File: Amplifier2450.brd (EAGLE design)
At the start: 28.2 x 35.5 mm, 17 parts, among them X1 SMA-142-0701-801/806, X2 SMA-142-0701-801/806

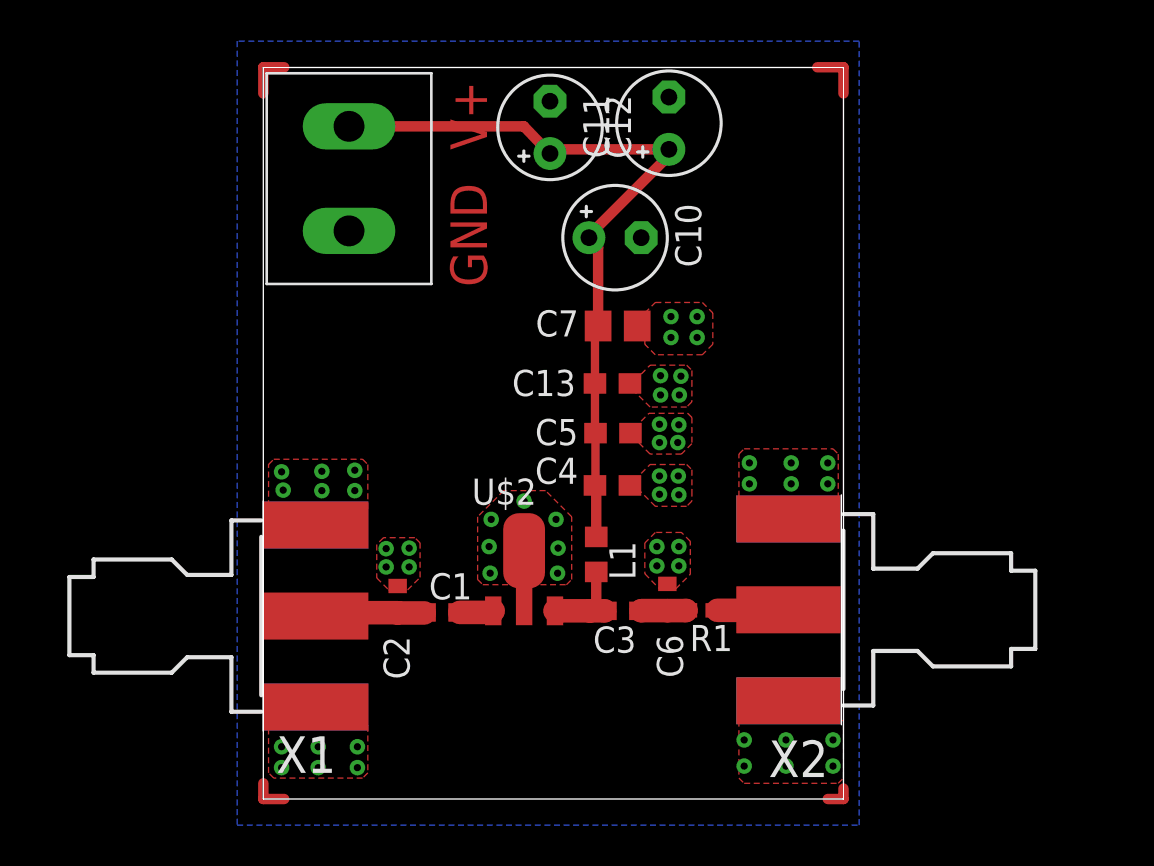
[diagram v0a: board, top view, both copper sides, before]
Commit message: (Tobias): made finishing touches to the design
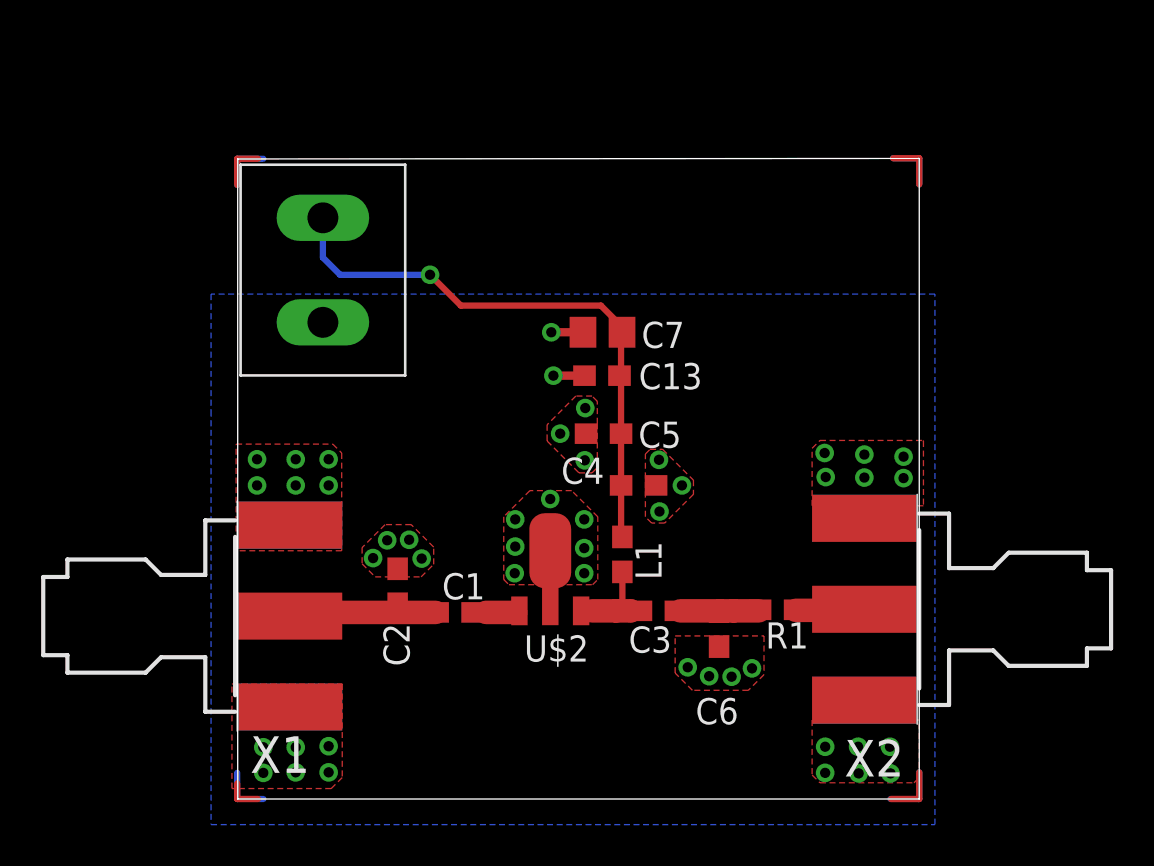
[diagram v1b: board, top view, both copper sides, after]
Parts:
- removed C10, C11, C12: 10u, rcl:E2,5-5
- C1, C2, C3, C6: device rcl:C0402 -> rcl:C0603
- L1: device own_htl3r-discrete-1:R_SMD0603 -> rcl:C0603
- R1: device rcl:R0402 -> rcl:C0603
- moved U$1 4.62 mm to (2.90, 25.7)
- moved R1 3.71 mm to (25.0, 9.19)
- moved X2 3.68 mm to (31.8, 9.22)
- moved C6 2.95 mm to (22.1, 8.26), turned to 270 degrees
- moved C3 1.73 mm to (19.2, 9.14)
- moved C4 1.27 mm to (18.2, 15.2)
- moved X1 1.27 mm to (-1.27, 8.89)
- moved L1 1.27 mm to (17.4, 11.9)
- moved U$2 1.27 mm to (13.9, 11.1)
- moved C7 0.80 mm to (16.5, 22.7), turned to 180 degrees
- moved C1 0.63 mm to (9.32, 9.07)
- moved C2 0.63 mm to (6.53, 10.3)
- moved C13 0.63 mm to (16.5, 20.6), turned to 180 degrees
- moved C5 0.46 mm to (16.5, 17.8), turned to 180 degrees
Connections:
- net +5V: no longer C10.+, C11.+, C12.+
- net GND: no longer C10.-, C11.-, C12.-
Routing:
- net +5V: track 37.4 -> 28.3 mm, vias 0 -> 1
- net GND: track 1.60 -> 4.65 mm, vias 55 -> 47
- net N$13: track 0.00 -> 2.69 mm
- net N$12: track 0.00 -> 2.54 mm
- net N$14: track 0.00 -> 2.54 mm
- net N$4: track 2.35 -> 4.80 mm
- net N$2: track 5.78 -> 7.74 mm
- net N$3: track 1.66 -> 3.39 mm
- net N$7: track 1.27 -> 2.67 mm
- net N$16: track 0.00 -> 1.27 mm
- net N$15: track 0.00 -> 1.24 mm
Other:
- board size 28.2 x 35.5 mm -> 33.1 x 31.1 mm
- board text added: "* Power line width at 12mil resulting Impedance is ~98Ohm * Power Reflectance to the signal line is about 10% = ((Z_s - Z_p) / (Z_s - Z_p))^2 * Heat increase of the powerline at 130mA will be less than 2 Kelvin"
- board text added: "Disable thermals around pads and vias, because they would introduce additional small wire inductors."
- board text added: "Have power lines close to each other to reduce noise captured in their spanning area"
- board text added: "Measurements are im mm"
- board text added: "Multiple vias on C4 and C5, event though they are only at DC, to reduce the inductive effects because they have very small capazitive values"
- board text added: "Spread Vias around C6 for sliding"
- board text removed: "?????????? Can we use a different width for the power line, so that it has a different impedance and RF will not go up the power line because it would be reflected."
- board text removed: "GND"
- board text removed: "Starpoint of the power planes/lines to minimize potential loop area."
- board text removed: "V+"
